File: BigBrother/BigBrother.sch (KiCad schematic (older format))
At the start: 4 parts

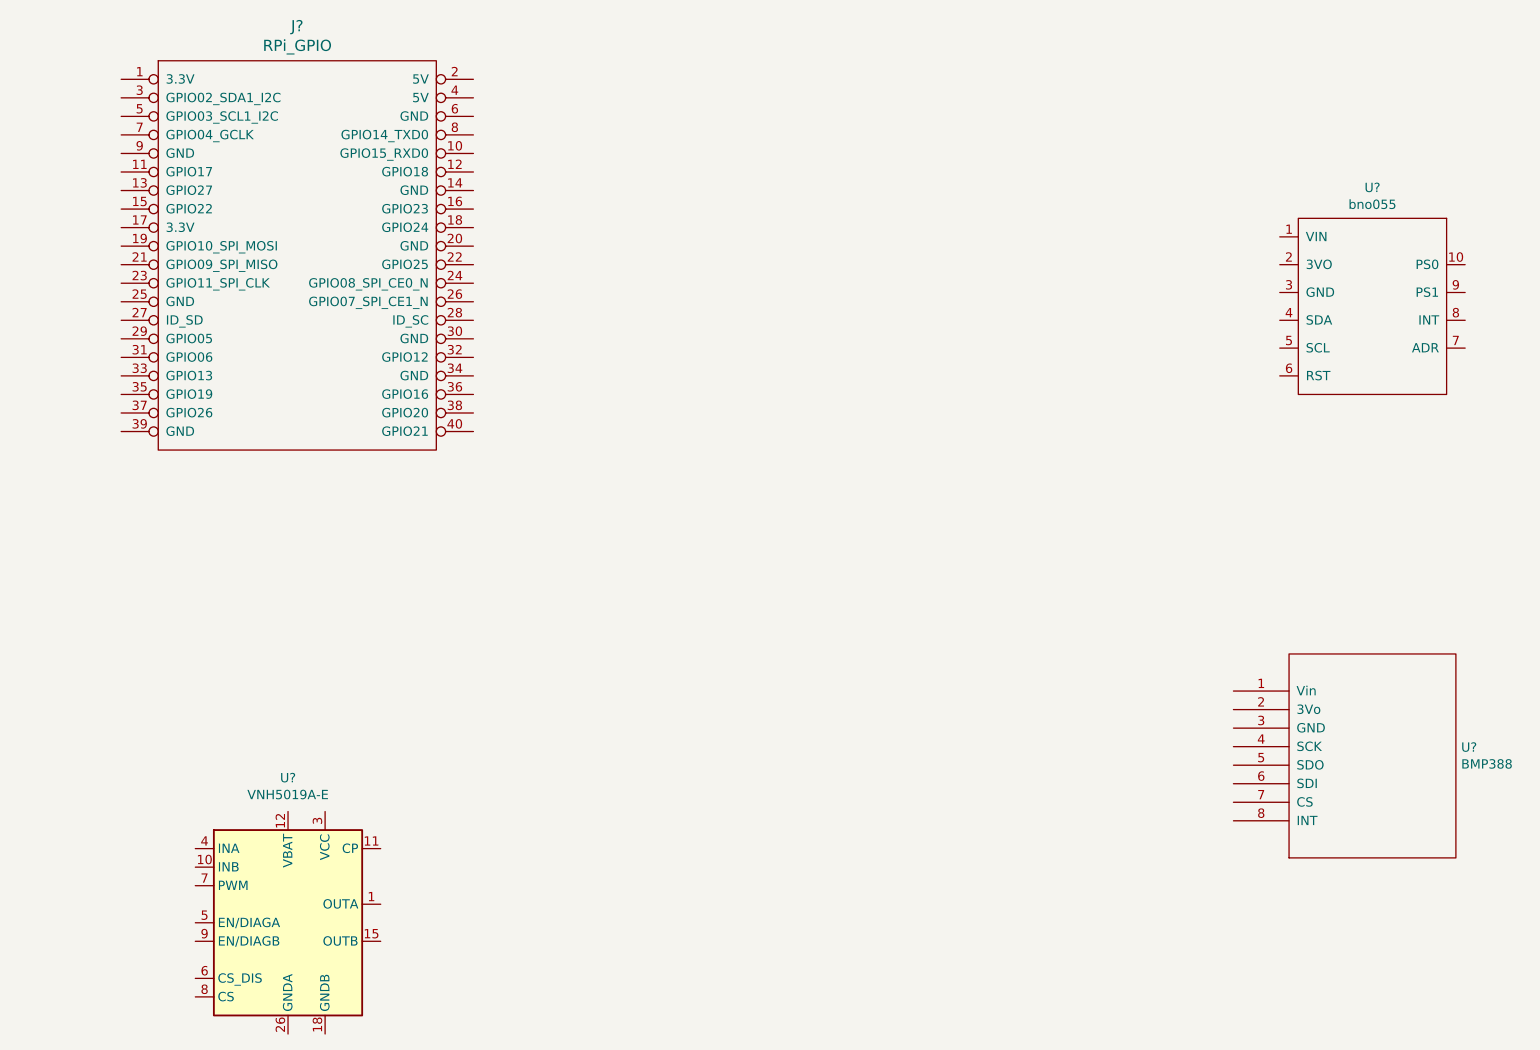
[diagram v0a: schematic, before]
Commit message: BigBrother Update
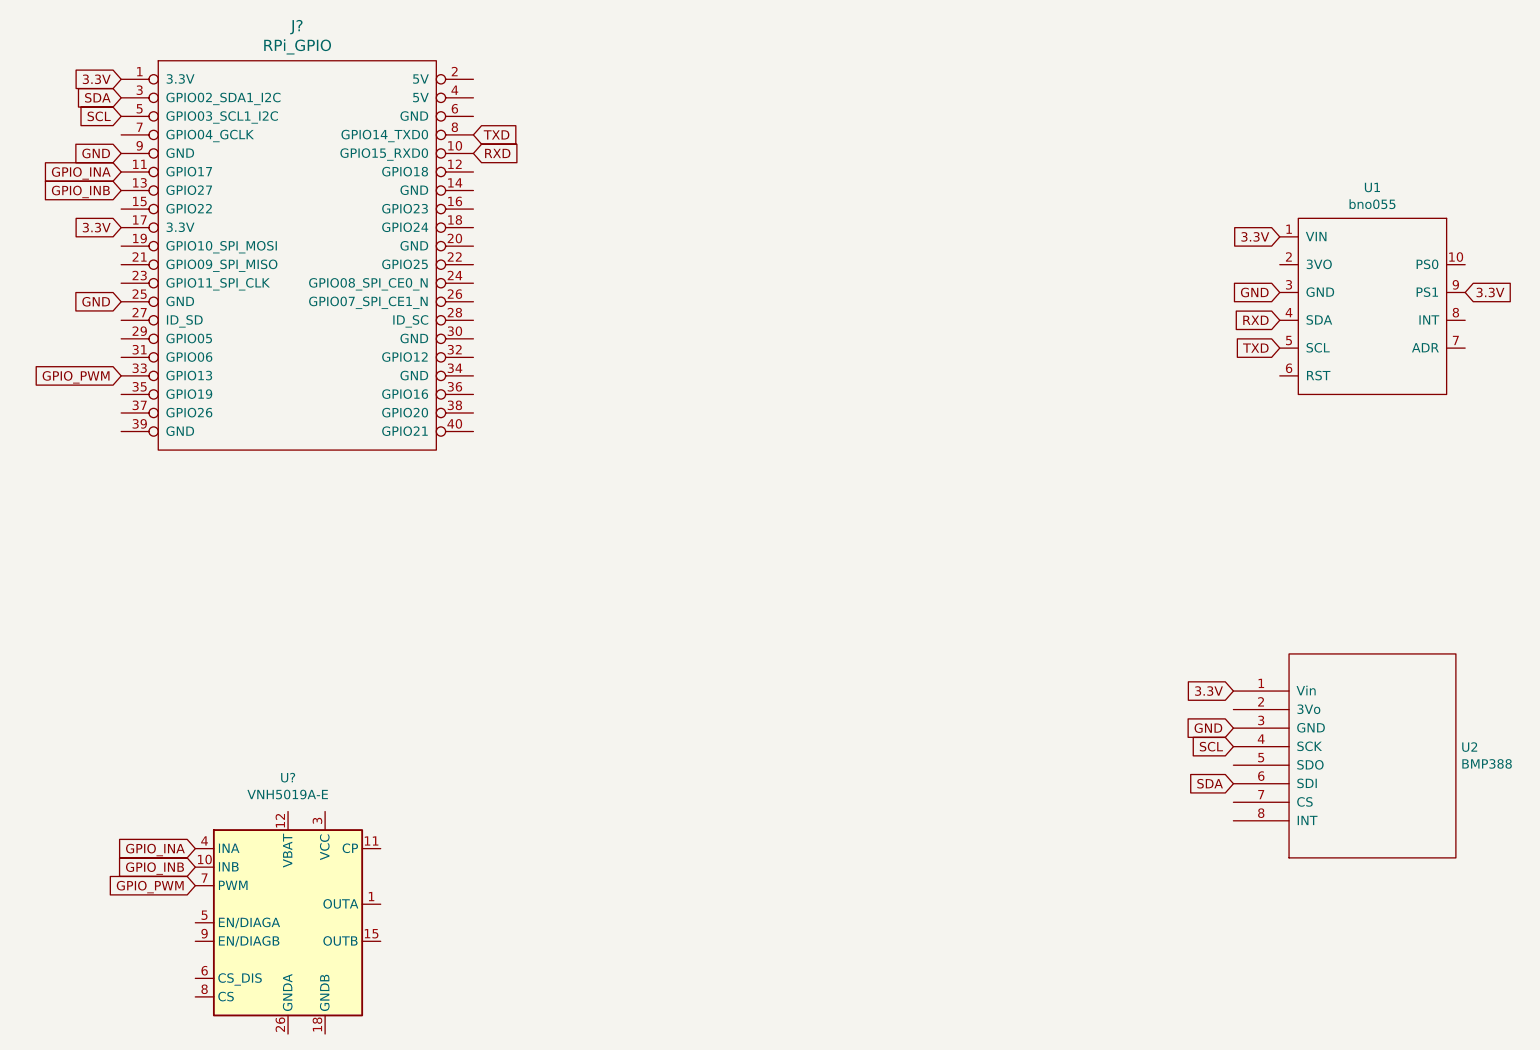
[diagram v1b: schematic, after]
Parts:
- gave numbers to parts that had none: 2
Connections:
- net 3.3V: now reaches J?.1 (3.3V)
- net 3.3V: now also J?.17 (3.3V), U1.1 (VIN), U1.9 (PS1), U2.1 (Vin)
- net RXD: now reaches J?.10 (GPIO15_RXD0)
- net RXD: now also U1.4 (SDA)
- net GPIO_INA: now reaches J?.11 (GPIO17)
- net GPIO_INA: now also U?.4 (INA)
- net GPIO_INB: now reaches J?.13 (GPIO27)
- net GPIO_INB: now also U?.10 (INB)
- net GND: now reaches J?.25 (GND)
- net GND: now also J?.9 (GND), U1.3 (GND), U2.3 (GND)
- net SDA: now reaches J?.3 (GPIO02_SDA1_I2C)
- net SDA: now also U2.6 (SDI)
- net GPIO_PWM: now reaches J?.33 (GPIO13)
- net GPIO_PWM: now also U?.7 (PWM)
- net SCL: now reaches J?.5 (GPIO03_SCL1_I2C)
- net SCL: now also U2.4 (SCK)
- net TXD: now reaches J?.8 (GPIO14_TXD0)
- net TXD: now also U1.5 (SCL)
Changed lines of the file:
@@
 $EndComp
 $Comp
-L bno055-breakout:bno055 U?
+L BMP388:BMP388 U2
+U 1 1 5E48BA81
+P 8300 5000
+F 0 "U2" H 8778 5046 50  0000 L CNN
+F 1 "BMP388" H 8778 4955 50  0000 L CNN
+F 2 "MODULE" H 8300 5000 50  0001 C CNN
+F 3 "DOCUMENTATION" H 8300 5000 50  0001 C CNN
+	1    8300 5000
+	1    0    0    -1
+$EndComp
+Text GLabel 1550 1350 0    50   Input ~ 0
+3.3V
+Text GLabel 1550 1750 0    50   Input ~ 0
+GND
+Text GLabel 3450 1750 2    50   Input ~ 0
+RXD
+Text GLabel 7800 2500 0    50   Input ~ 0
+GND
+Text GLabel 7800 2200 0    50   Input ~ 0
+3.3V
+$Comp
+L bno055-breakout:bno055 U1
 U 1 1 5E48AFB4
 P 7900 2100
-F 0 "U?" H 8300 2265 50  0000 C CNN
+F 0 "U1" H 8300 2265 50  0000 C CNN
 F 1 "bno055" H 8300 2174 50  0000 C CNN
 F 2 "" H 8250 2250 50  0001 C CNN
@@
 	1    0    0    -1
 $EndComp
-$Comp
-L BMP388:BMP388 U?
-U 1 1 5E48BA81
-P 8300 5000
-F 0 "U?" H 8778 5046 50  0000 L CNN
-F 1 "BMP388" H 8778 4955 50  0000 L CNN
-F 2 "MODULE" H 8300 5000 50  0001 C CNN
-F 3 "DOCUMENTATION" H 8300 5000 50  0001 C CNN
-	1    8300 5000
-	1    0    0    -1
-$EndComp
+Text GLabel 7800 2650 0    50   Input ~ 0
+RXD
+Text GLabel 3450 1650 2    50   Input ~ 0
+TXD
+Text GLabel 7800 2800 0    50   Input ~ 0
+TXD
+Text GLabel 8800 2500 2    50   Input ~ 0
+3.3V
+Text GLabel 1550 2150 0    50   Input ~ 0
+3.3V
+Text GLabel 7550 4650 0    50   Input ~ 0
+3.3V
+Text GLabel 1550 2550 0    50   Input ~ 0
+GND
+Text GLabel 7550 4850 0    50   Input ~ 0
+GND
+Text GLabel 1550 1550 0    50   Input ~ 0
+SCL
+Text GLabel 7550 4950 0    50   Input ~ 0
+SCL
+Text GLabel 1550 1450 0    50   Input ~ 0
+SDA
+Text GLabel 7550 5150 0    50   Input ~ 0
+SDA
+Text GLabel 1550 2950 0    50   Input ~ 0
+GPIO_PWM
+Text GLabel 1950 5700 0    50   Input ~ 0
+GPIO_PWM
+Text GLabel 1550 1850 0    50   Input ~ 0
+GPIO_INA
+Text GLabel 1950 5500 0    50   Input ~ 0
+GPIO_INA
+Text GLabel 1550 1950 0    50   Input ~ 0
+GPIO_INB
+Text GLabel 1950 5600 0    50   Input ~ 0
+GPIO_INB
 $EndSCHEMATC
